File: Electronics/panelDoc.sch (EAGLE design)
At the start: 35 parts

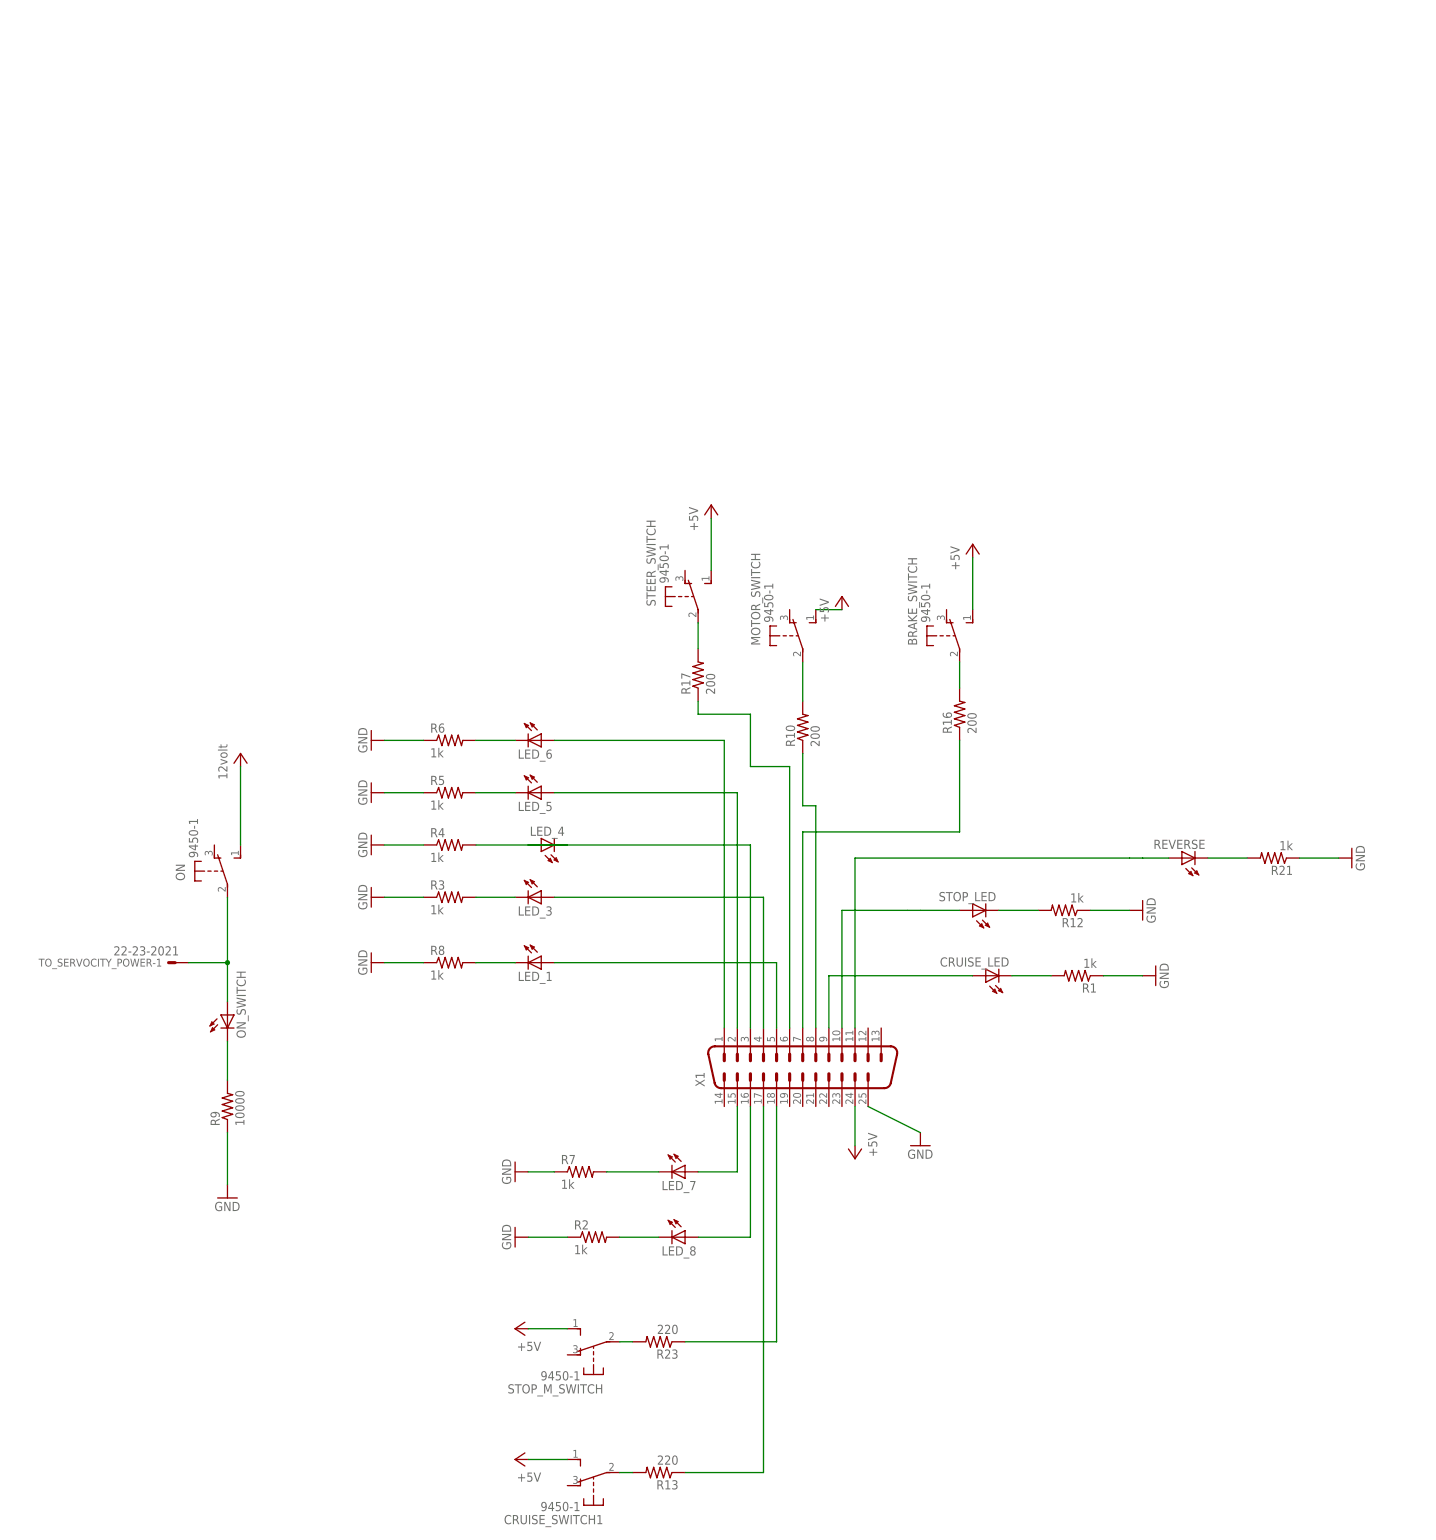
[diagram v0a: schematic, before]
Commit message: Diagram made neater.
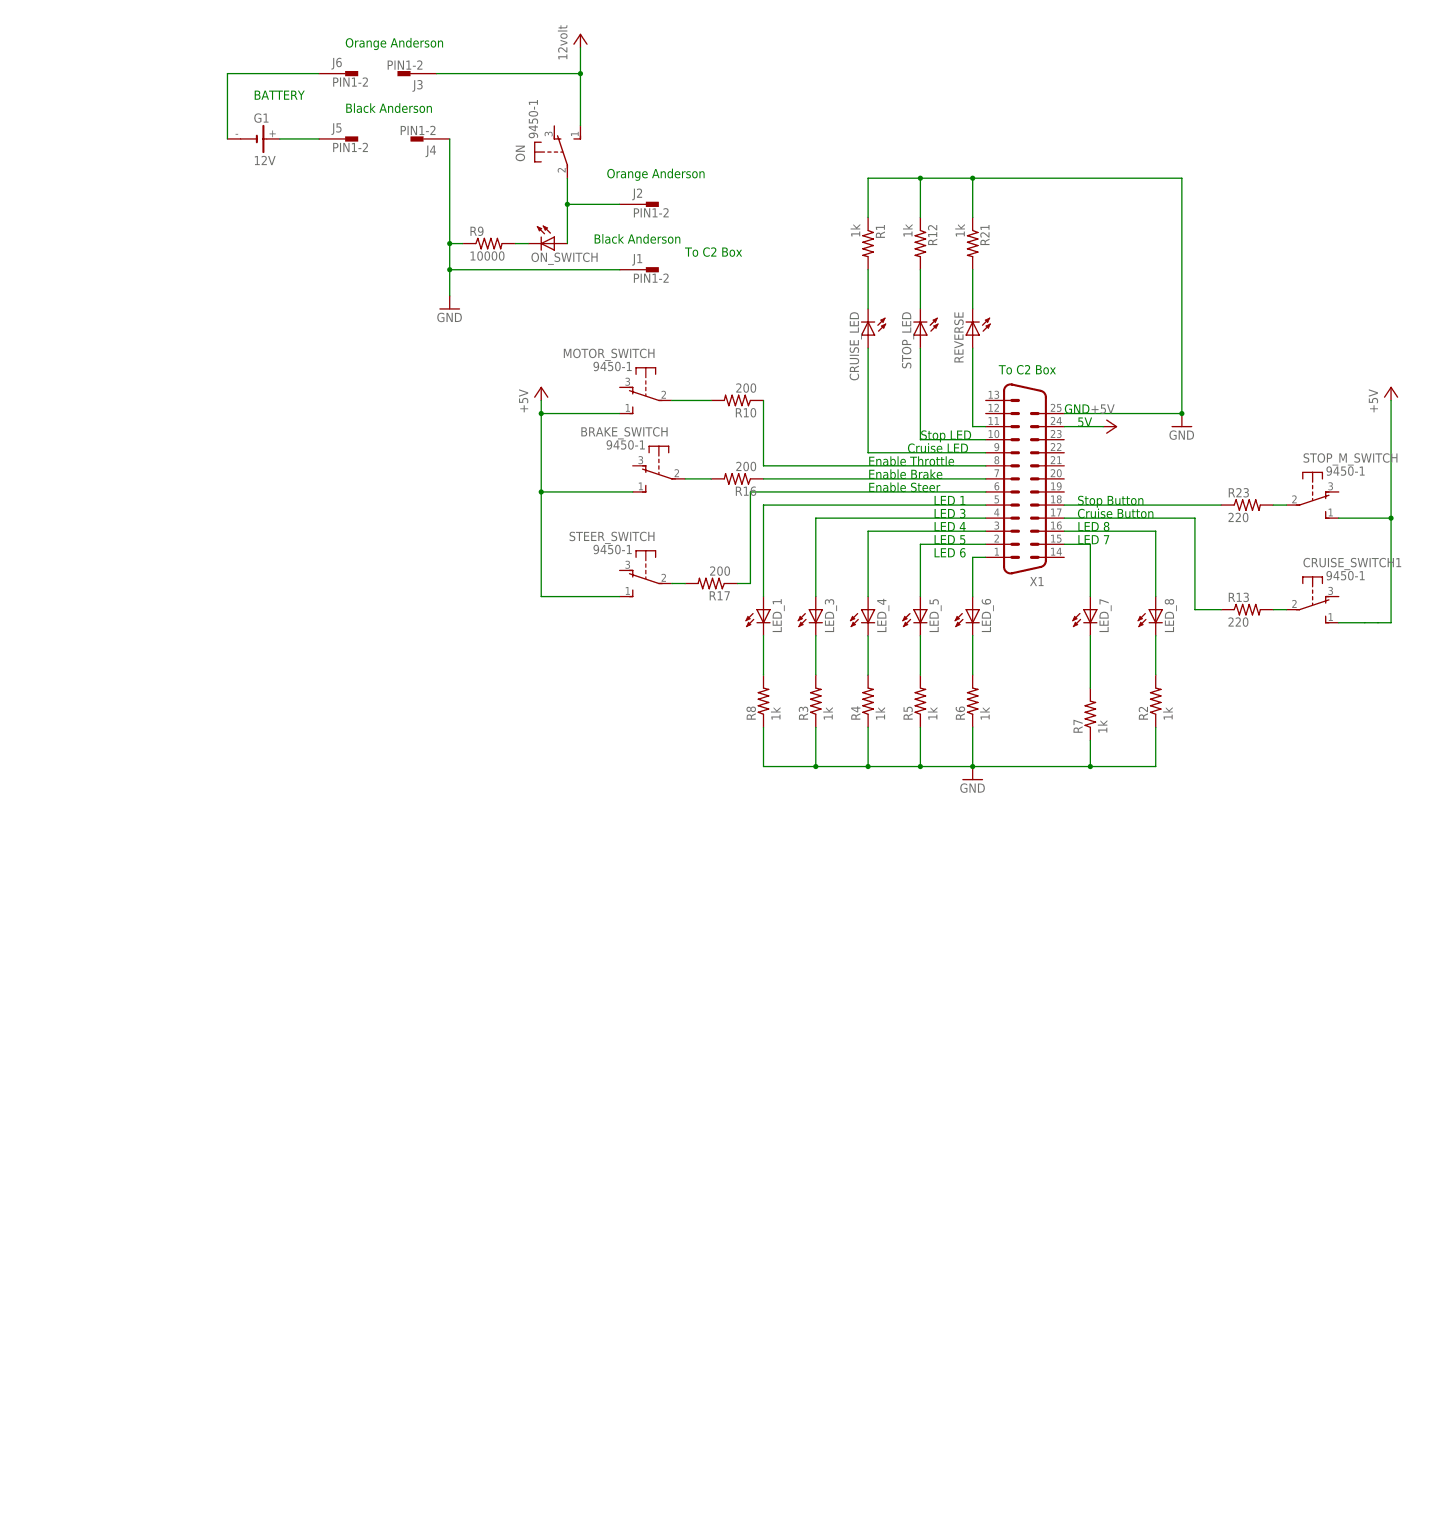
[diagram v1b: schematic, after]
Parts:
- removed TO_SERVOCITY_POWER: 22-23-2021, con-molex:22-23-2021
- added G1: 12V, battery:SL-150-1/2AA/PT
- added J1, J2, J3, J4, J5, J6: PIN1-2, con-faston:PIN1-2
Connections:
- new net N$21: G1.-, J6.1
- new net N$23: G1.+, J5.1
- net +5V: now also J3.1
- net GND: now also J1.1, J4.1
- net N$17: now also J2.1; no longer TO_SERVOCITY_POWER-1.S
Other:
- note added: "5V"
- note added: "BATTERY"
- note added: "Black Anderson"
- note added: "Cruise Button"
- note added: "Cruise LED"
- note added: "Enable Brake"
- note added: "Enable Steer"
- note added: "Enable Throttle"
- note added: "GND"
- note added: "LED 1"
- note added: "LED 3"
- note added: "LED 4"
- note added: "LED 5"
- note added: "LED 6"
- note added: "LED 7"
- note added: "LED 8"
- note added: "Orange Anderson"
- note added: "Stop Button"
- note added: "Stop LED"
- note added: "To C2 Box"
- moved on the sheet: BRAKE_SWITCH, CRUISE_LED, CRUISE_SWITCH1, LED_1, LED_3, LED_4, LED_5, LED_6, LED_7, LED_8, MOTOR_SWITCH, ON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
